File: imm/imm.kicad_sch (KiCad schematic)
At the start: 15 parts, among them J1 Conn_01x02, J2 Conn_01x03, Q1 D4184, U1 EL817

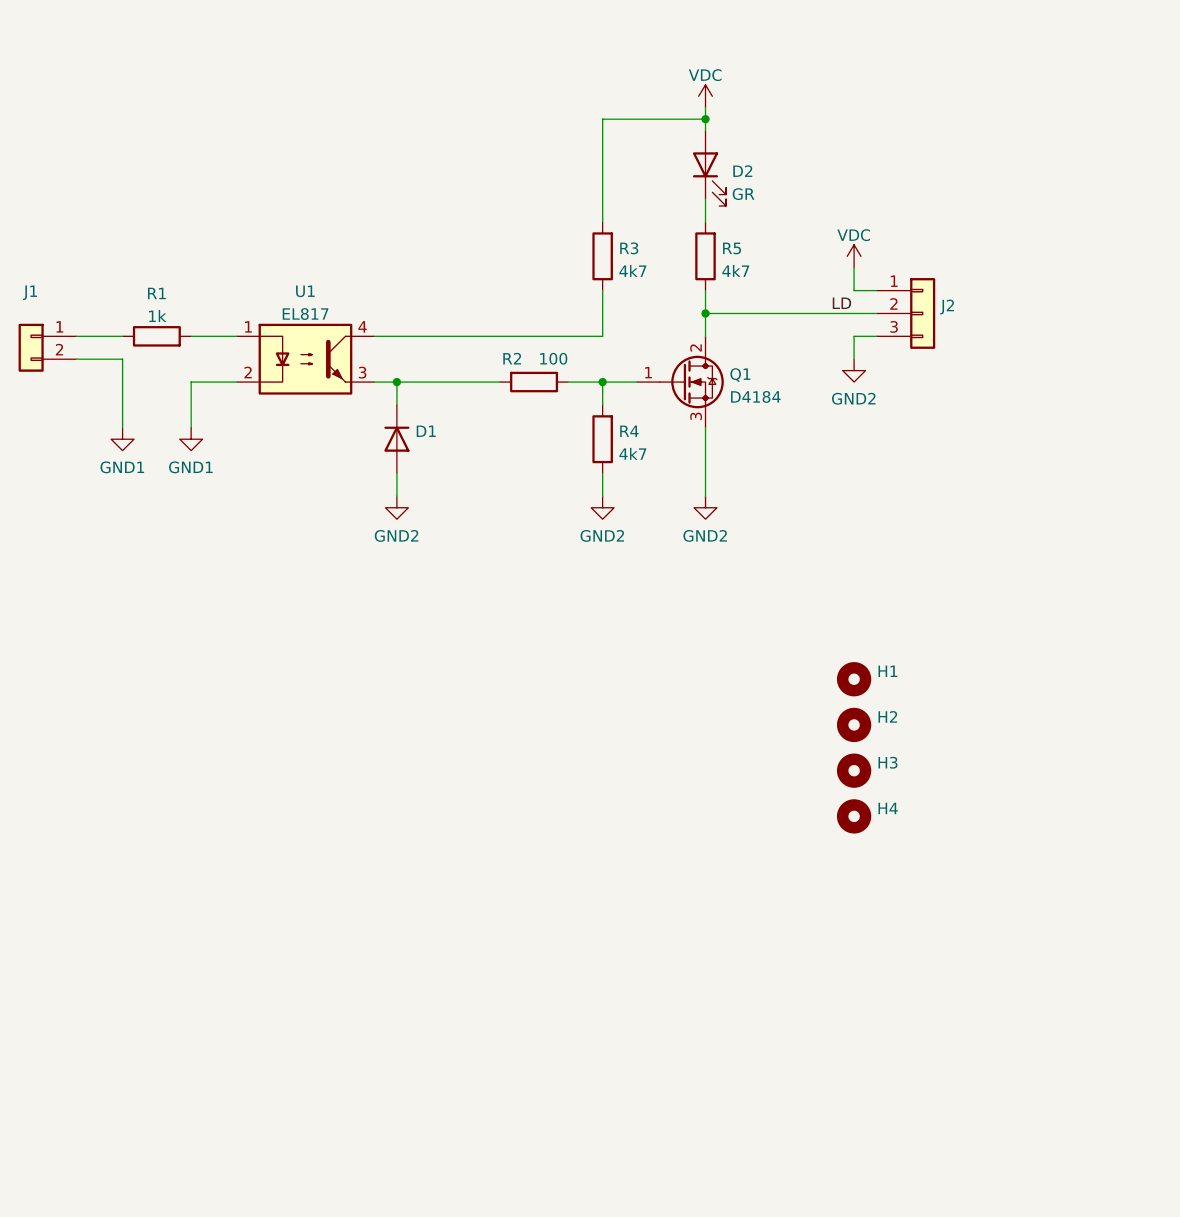
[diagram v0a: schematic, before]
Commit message: Hmmm
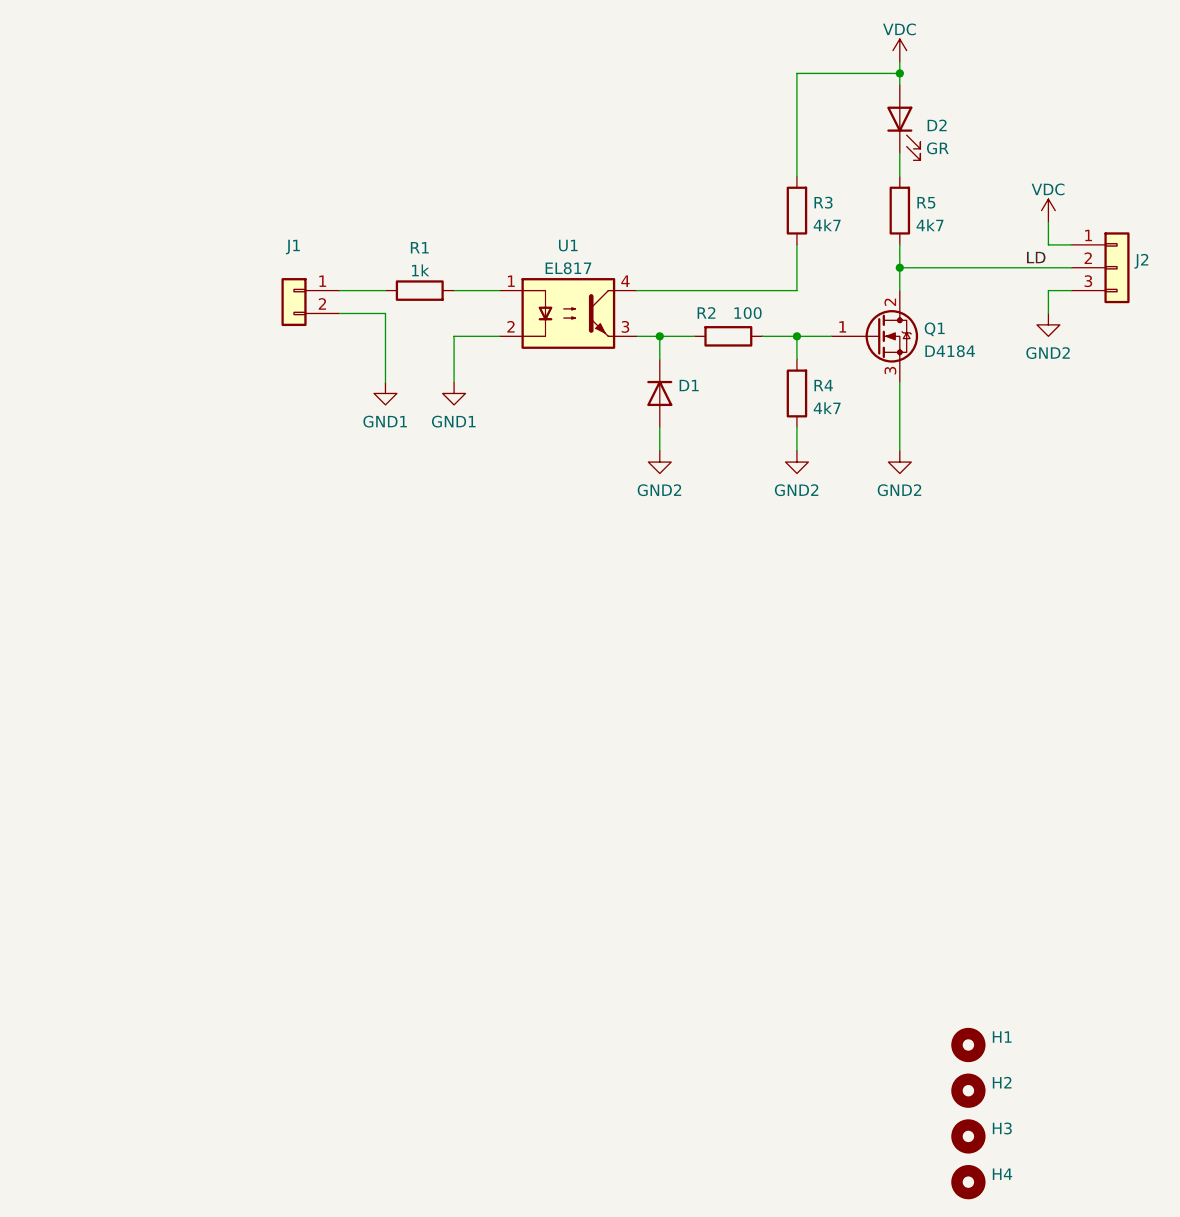
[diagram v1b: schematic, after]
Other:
- moved on the sheet: D1, D2, H1, H2, H3, H4, J1, J2, Q1, R1, R2, R3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
